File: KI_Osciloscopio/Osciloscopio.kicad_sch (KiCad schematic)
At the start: 46 parts, among them CN1 Conector IZQ, CN2 Conector DER, J1 Barrel Jack, J2 Conn_Coaxial, J3 OLED 128x64, J4 USB_B, U1 MCP6004, U2 74HC4051, U3 LM2940CT-5.0/NOPB, U4 LM1117-3.3, U5 M95128

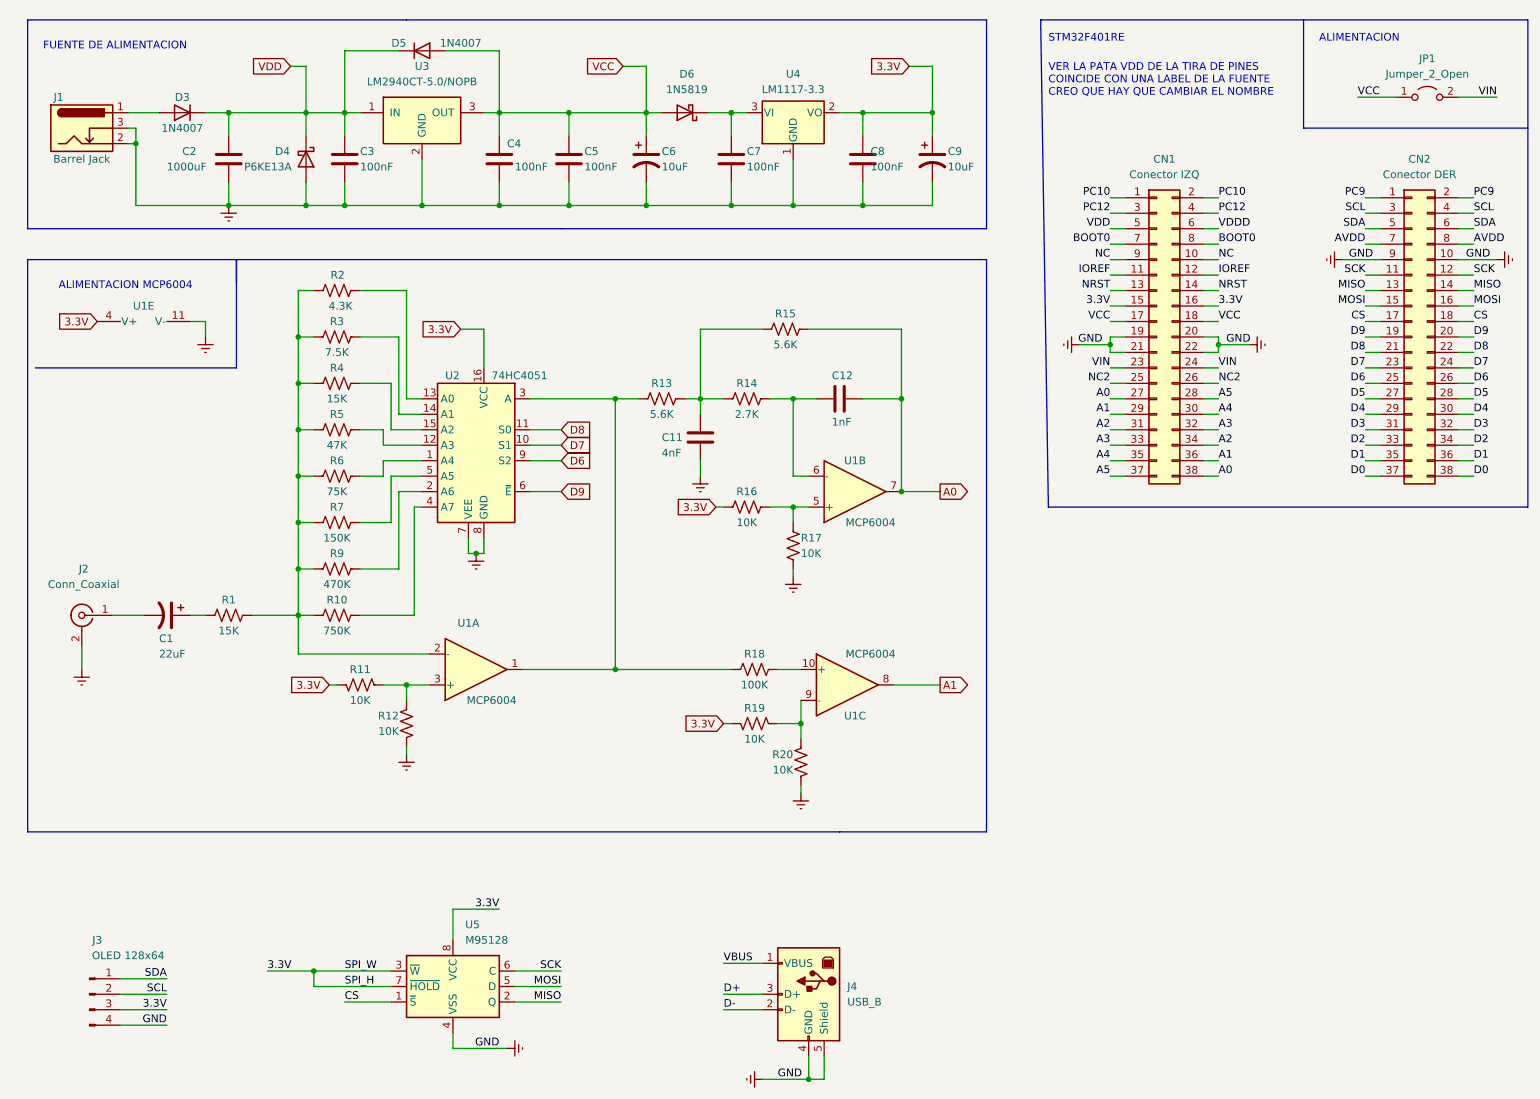
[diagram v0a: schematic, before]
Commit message: Cambie el circuito de alimentacion
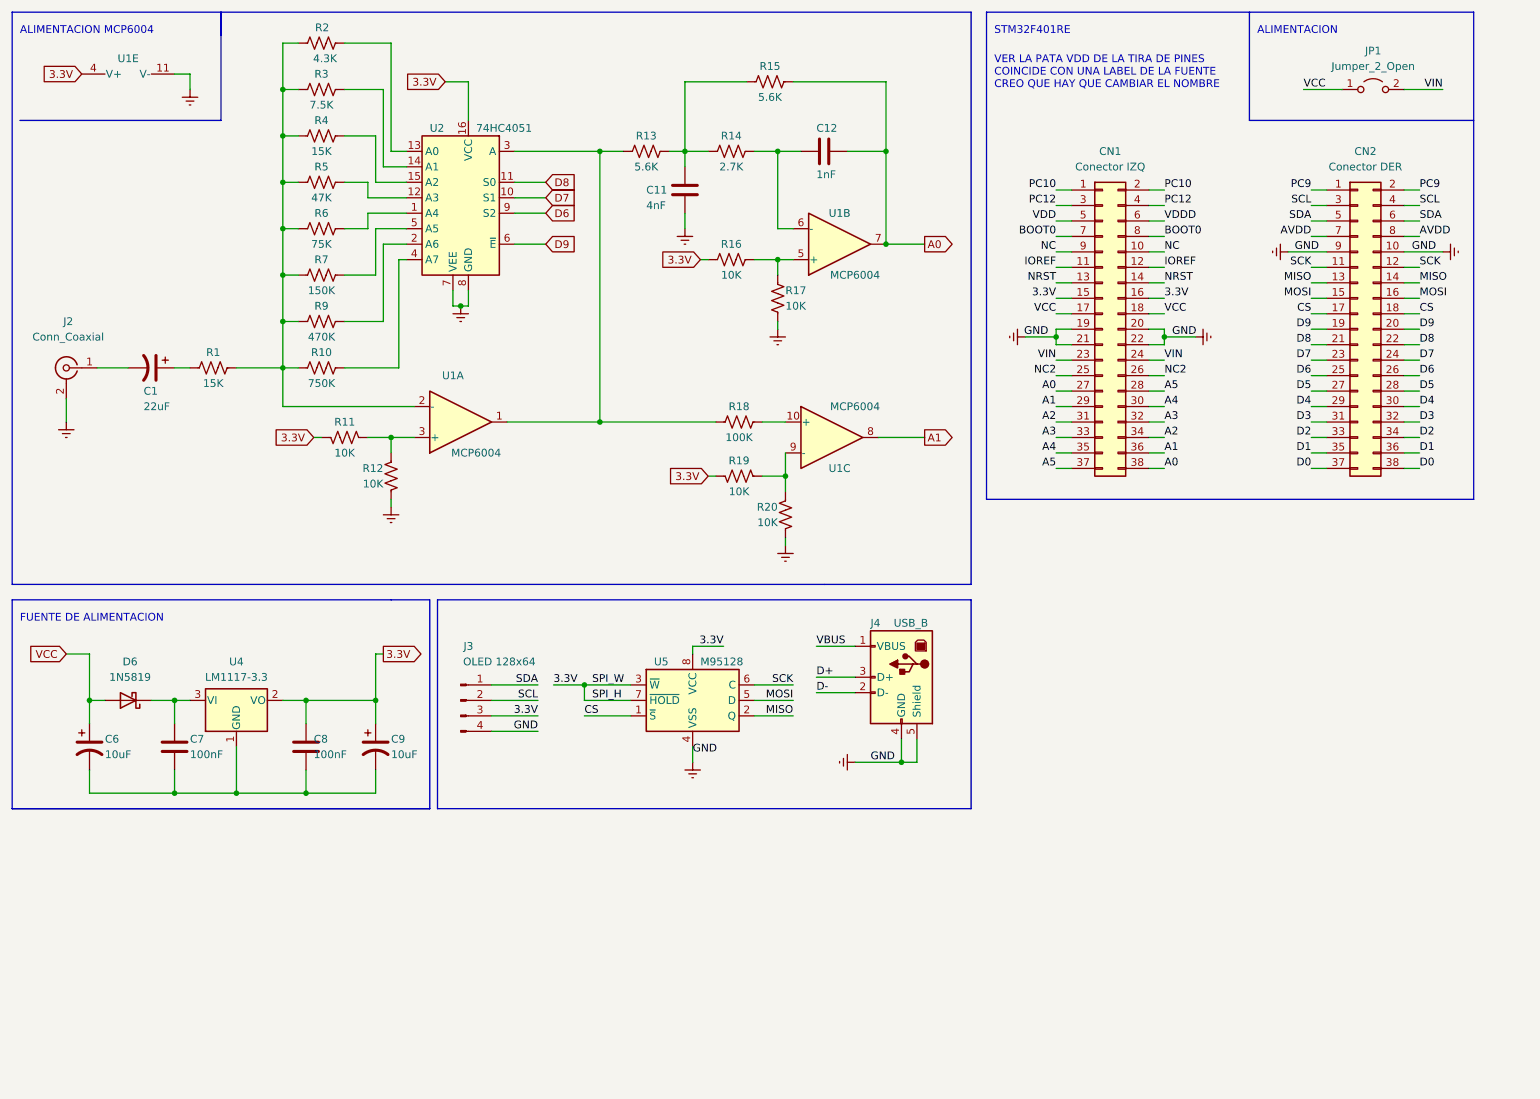
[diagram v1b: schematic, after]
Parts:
- removed C2: 1000uF, Capacitor_THT:C_Disc_D5.0mm_W2.5mm_P2.50mm, symbol Device:C
- removed C3, C4, C5: 100nF, Capacitor_THT:C_Disc_D5.0mm_W2.5mm_P2.50mm, symbol Device:C
- removed D3, D5: 1N4007, Diode_THT:D_DO-41_SOD81_P10.16mm_Horizontal, symbol Diode:1N4007
- removed D4: P6KE13A, Diode_THT:D_DO-15_P10.16mm_Horizontal, symbol Device:D_Schottky
- removed J1: Barrel Jack, Connector_BarrelJack:BarrelJack_Horizontal, symbol Connector:Barrel_Jack_Switch
- removed U3: LM2940CT-5.0/NOPB, Package_TO_SOT_THT:TO-220-3_Vertical, symbol AOI-LM2940CT:LM2940CT-5.0/NOPB
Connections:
- net Earth: no longer C6.2, C7.2, C8.2, C9.2, U4.1 (GND)
- new net: C6.2, C7.2, C8.2, C9.2, U4.1 (GND)
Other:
- moved on the sheet: C1, C11, C12, C6, C7, C8, C9, CN1, CN2, D6, J2, J3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
